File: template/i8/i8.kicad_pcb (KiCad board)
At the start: 2 copper layers, 50 x 50 mm, 32 parts, among them J1 ZX-SH1.0-4PWT, J2 Conn_DEBUG, U1 XC6206P332MR-G, U2 RP2040, U3 W25Q16JVUXIQ, Y1 Crystal_GND24

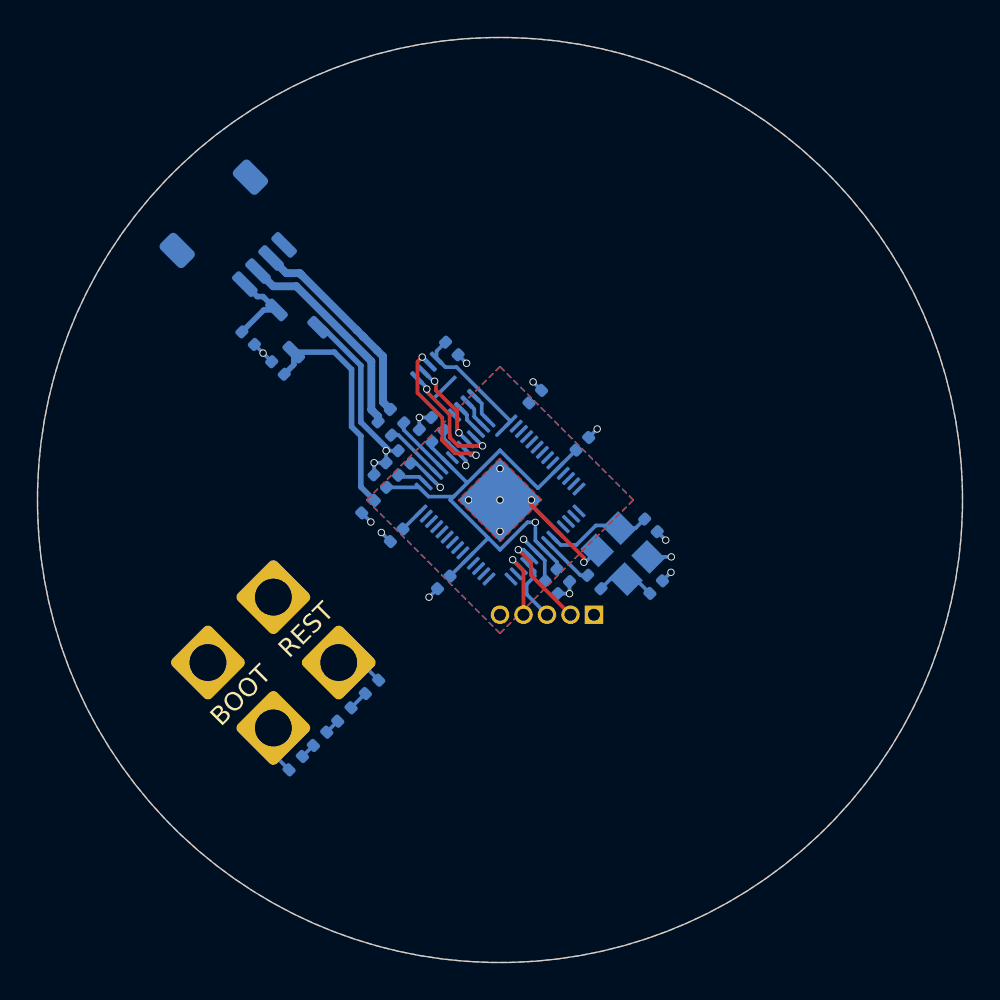
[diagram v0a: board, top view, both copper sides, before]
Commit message: i8 development
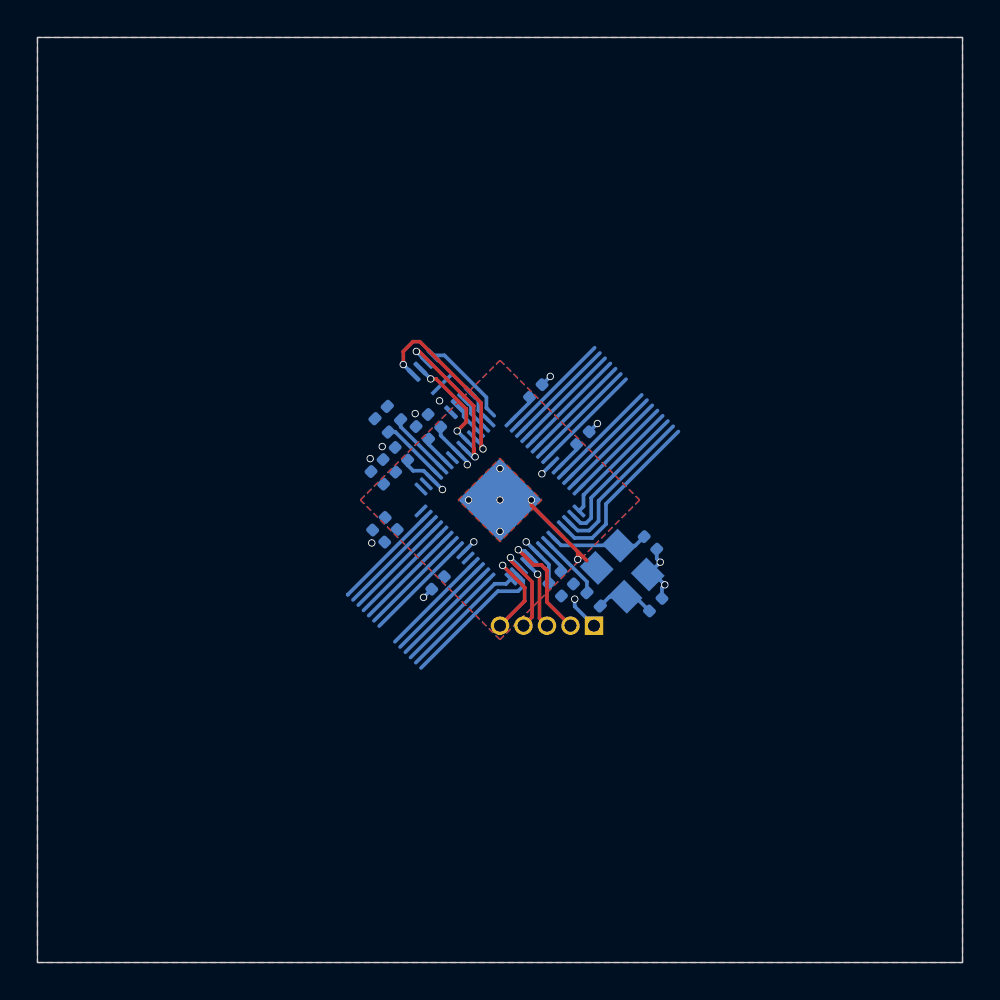
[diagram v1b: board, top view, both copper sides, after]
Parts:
- removed C13, C14, C15: 1u, Capacitor_SMD:C_0402_1005Metric
- removed J1: ZX-SH1.0-4PWT, Connector_JST:JST_SH_SM04B-SRSS-TB_1x04-1MP_P1.00mm_Horizontal
- removed PSW1: REST, i8:JUMP_1x2
- removed PSW2: BOOT, i8:JUMP_1x2
- removed R3, R5, R6: 5.1k, Resistor_SMD:R_0402_1005Metric
- removed R7: 1k, Resistor_SMD:R_0402_1005Metric
- removed U1: XC6206P332MR-G, Package_TO_SOT_SMD:SOT-23-3
- C1, C10, C11, C12, C16, C17, C2, C3, C4, C5, C6, C7, C8, C9: footprint Capacitor_SMD:C_0402_1005Metric -> i8:C_0402_1005Metric_mod
- moved C2 11.0 mm to (-3.55, -4.28), turned to 135 degrees
- moved C3 11.0 mm to (2.98, 4.85), turned to -45 degrees
- moved C4 1.10 mm to (-6.54, 1.28)
- moved C16 0.95 mm to (8.13, 2.32)
- moved Y1 0.95 mm to (6.61, 3.85)
- moved C17 0.95 mm to (8.42, 5.66)
- moved R4 0.94 mm to (5.06, 5.37)
- moved J2 0.59 mm to (5.08, 6.79)
- moved C9 0.31 mm to (-3.35, 4.48)
- moved C10 0.31 mm to (-5.89, 1.93)
- moved C7 0.31 mm to (4.48, -3.35)
- moved C6 0.31 mm to (1.93, -5.89)
- moved C8 0.24 mm to (3.63, 4.20)
- moved C1 0.24 mm to (-5.33, -2.50)
- moved U3 0.24 mm to (-3.13, -6.28)
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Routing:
- net +3V3: track 52.5 -> 16.1 mm
- net GND: track 29.1 -> 14.0 mm, vias 20 -> 17
- net D-: track 11.6 -> 0.00 mm
- net D+: track 11.3 -> 0.00 mm
- net GPIO15: track 0.00 -> 9.50 mm
- net GPIO14: track 0.00 -> 8.84 mm
- net GPIO16: track 0.00 -> 8.18 mm
- net GPIO13: track 0.00 -> 8.18 mm
- net GPIO12: track 0.00 -> 7.02 mm
- net GPIO17: track 0.00 -> 7.02 mm
- net GPIO5: track 0.00 -> 6.00 mm
- net GPIO11: track 0.00 -> 6.00 mm
- net GPIO6: track 0.00 -> 6.00 mm
- net GPIO29_ADC3: track 0.00 -> 6.00 mm
- net GPIO24: track 0.00 -> 6.00 mm
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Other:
- outline, holes or cut-outs redrawn
- board text added: "copper .9mm"
- board text added: "via"
- board text added: "zone"
